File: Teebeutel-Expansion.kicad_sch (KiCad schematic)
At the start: 63 parts, among them J1 Conn_01x10_Male, J2 Conn_01x10_Female, J3 Conn_01x10_Male, J4 Conn_01x10_Female, J5 Conn_02x03_Counter_Clockwise, J6 Conn_02x03_Counter_Clockwise, J7 Conn_01x03, J8 Conn_01x03, J9 Conn_02x08_Counter_Clockwise

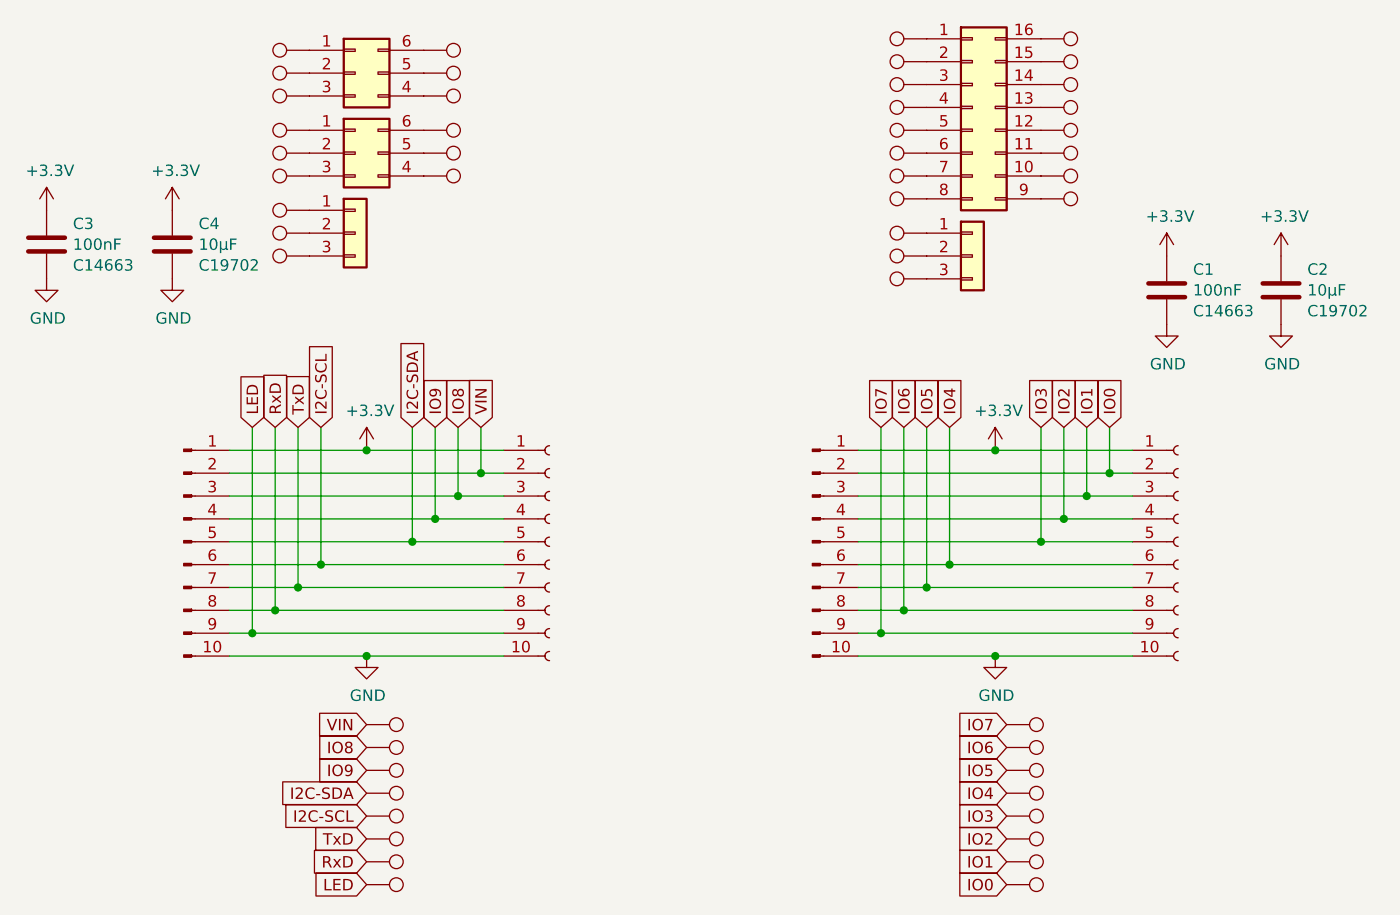
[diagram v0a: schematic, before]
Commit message: chore: Update labels
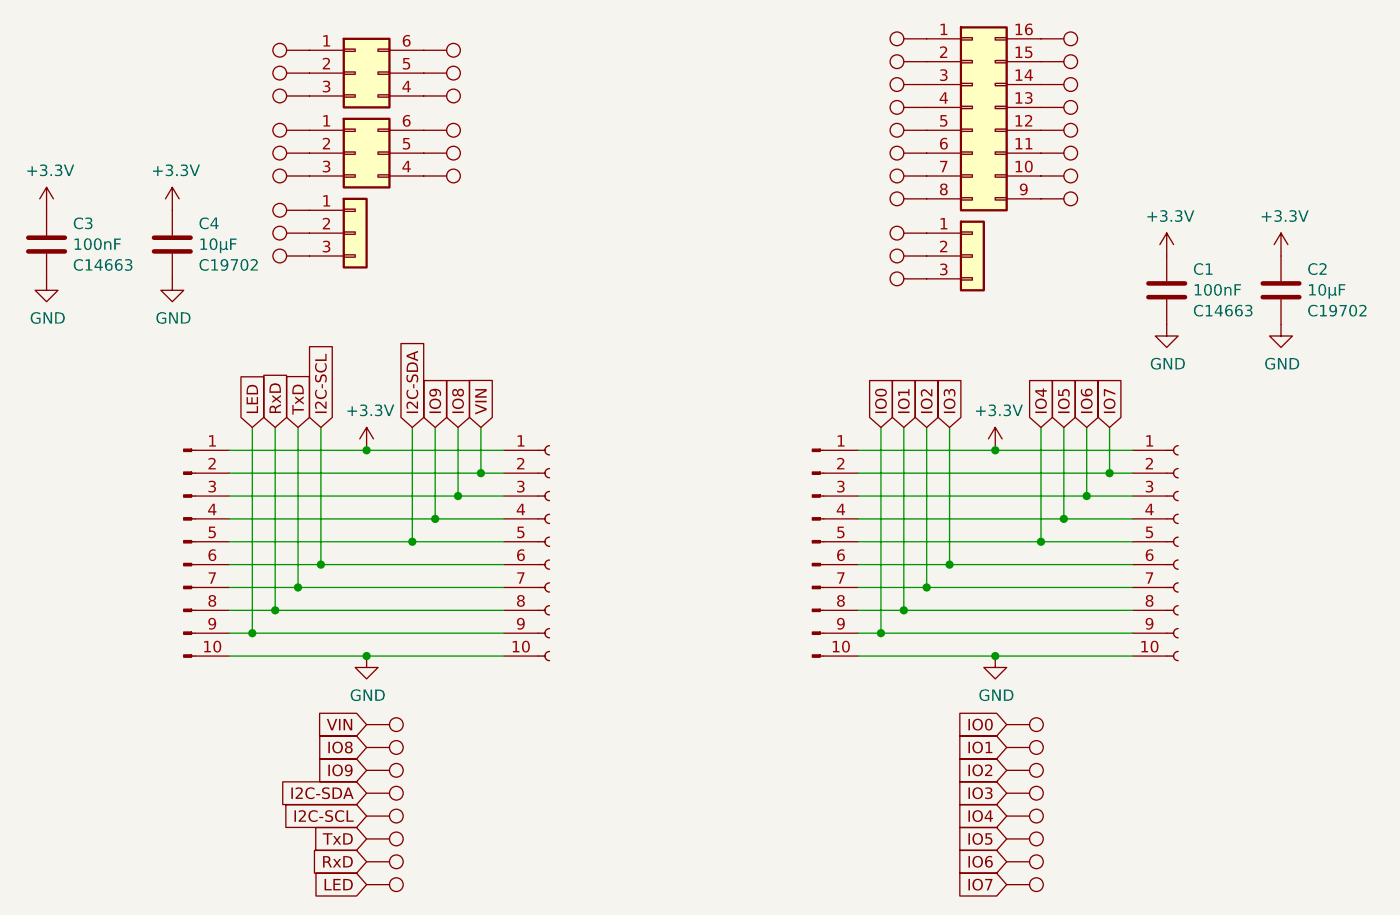
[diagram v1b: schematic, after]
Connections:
- net IO0: now also J3.9 (Pin_9), J4.9 (Pin_9), TP16.1; no longer J3.2 (Pin_2), J4.2 (Pin_2), TP9.1
- net IO1: now also J3.8 (Pin_8), J4.8 (Pin_8), TP15.1; no longer J3.3 (Pin_3), J4.3 (Pin_3), TP10.1
- net IO2: now also J3.7 (Pin_7), J4.7 (Pin_7), TP14.1; no longer J3.4 (Pin_4), J4.4 (Pin_4), TP11.1
- net IO3: now also J3.6 (Pin_6), J4.6 (Pin_6), TP13.1; no longer J3.5 (Pin_5), J4.5 (Pin_5), TP12.1
- net IO4: now also J3.5 (Pin_5), J4.5 (Pin_5), TP12.1; no longer J3.6 (Pin_6), J4.6 (Pin_6), TP13.1
- net IO5: now also J3.4 (Pin_4), J4.4 (Pin_4), TP11.1; no longer J3.7 (Pin_7), J4.7 (Pin_7), TP14.1
- net IO6: now also J3.3 (Pin_3), J4.3 (Pin_3), TP10.1; no longer J3.8 (Pin_8), J4.8 (Pin_8), TP15.1
- net IO7: now also J3.2 (Pin_2), J4.2 (Pin_2), TP9.1; no longer J3.9 (Pin_9), J4.9 (Pin_9), TP16.1
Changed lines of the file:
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@@
     )
   )
-  (global_label "IO7" (shape input) (at 182.88 123.19 180) (fields_autoplaced)
+  (global_label "IO7" (shape input) (at 182.88 140.97 180) (fields_autoplaced)
     (effects (font (size 1.27 1.27)) (justify right))
-    (property "Intersheet References" "${INTERSHEET_REFS}" (id 0) (at 0 0 0)
+    (property "Intersheet References" "${INTERSHEET_REFS}" (id 0) (at 0 264.16 0)
       (effects (font (size 1.27 1.27)) hide)
     )
   )
-  (global_label "IO6" (shape input) (at 171.45 90.17 90) (fields_autoplaced)
+  (global_label "IO6" (shape input) (at 191.77 90.17 90) (fields_autoplaced)
     (effects (font (size 1.27 1.27)) (justify left))
-    (property "Intersheet References" "${INTERSHEET_REFS}" (id 0) (at 0 0 0)
+    (property "Intersheet References" "${INTERSHEET_REFS}" (id 0) (at 363.22 0 0)
       (effects (font (size 1.27 1.27)) hide)
     )
@@
     )
   )
-  (global_label "IO7" (shape input) (at 168.91 90.17 90) (fields_autoplaced)
+  (global_label "IO7" (shape input) (at 194.31 90.17 90) (fields_autoplaced)
     (effects (font (size 1.27 1.27)) (justify left))
-    (property "Intersheet References" "${INTERSHEET_REFS}" (id 0) (at 0 0 0)
+    (property "Intersheet References" "${INTERSHEET_REFS}" (id 0) (at 363.22 0 0)
       (effects (font (size 1.27 1.27)) hide)
     )
@@
     )
   )
-  (global_label "IO5" (shape input) (at 182.88 128.27 180) (fields_autoplaced)
+  (global_label "IO5" (shape input) (at 182.88 135.89 180) (fields_autoplaced)
     (effects (font (size 1.27 1.27)) (justify right))
-    (property "Intersheet References" "${INTERSHEET_REFS}" (id 0) (at 0 0 0)
+    (property "Intersheet References" "${INTERSHEET_REFS}" (id 0) (at 0 264.16 0)
       (effects (font (size 1.27 1.27)) hide)
     )
@@
     )
   )
-  (global_label "IO4" (shape input) (at 182.88 130.81 180) (fields_autoplaced)
+  (global_label "IO4" (shape input) (at 182.88 133.35 180) (fields_autoplaced)
     (effects (font (size 1.27 1.27)) (justify right))
-    (property "Intersheet References" "${INTERSHEET_REFS}" (id 0) (at 0 0 0)
+    (property "Intersheet References" "${INTERSHEET_REFS}" (id 0) (at 0 264.16 0)
       (effects (font (size 1.27 1.27)) hide)
     )
   )
-  (global_label "IO2" (shape input) (at 182.88 135.89 180) (fields_autoplaced)
+  (global_label "IO2" (shape input) (at 182.88 128.27 180) (fields_autoplaced)
     (effects (font (size 1.27 1.27)) (justify right))
-    (property "Intersheet References" "${INTERSHEET_REFS}" (id 0) (at 0 0 0)
+    (property "Intersheet References" "${INTERSHEET_REFS}" (id 0) (at 0 264.16 0)
       (effects (font (size 1.27 1.27)) hide)
     )
@@
     )
   )
-  (global_label "IO5" (shape input) (at 173.99 90.17 90) (fields_autoplaced)
+  (global_label "IO5" (shape input) (at 189.23 90.17 90) (fields_autoplaced)
     (effects (font (size 1.27 1.27)) (justify left))
-    (property "Intersheet References" "${INTERSHEET_REFS}" (id 0) (at 0 0 0)
+    (property "Intersheet References" "${INTERSHEET_REFS}" (id 0) (at 363.22 0 0)
       (effects (font (size 1.27 1.27)) hide)
     )
@@
     )
   )
-  (global_label "IO2" (shape input) (at 189.23 90.17 90) (fields_autoplaced)
+  (global_label "IO2" (shape input) (at 173.99 90.17 90) (fields_autoplaced)
     (effects (font (size 1.27 1.27)) (justify left))
-    (property "Intersheet References" "${INTERSHEET_REFS}" (id 0) (at 0 0 0)
+    (property "Intersheet References" "${INTERSHEET_REFS}" (id 0) (at 363.22 0 0)
       (effects (font (size 1.27 1.27)) hide)
     )
@@
     )
   )
-  (global_label "IO6" (shape input) (at 182.88 125.73 180) (fields_autoplaced)
+  (global_label "IO6" (shape input) (at 182.88 138.43 180) (fields_autoplaced)
     (effects (font (size 1.27 1.27)) (justify right))
-    (property "Intersheet References" "${INTERSHEET_REFS}" (id 0) (at 0 0 0)
+    (property "Intersheet References" "${INTERSHEET_REFS}" (id 0) (at 0 264.16 0)
       (effects (font (size 1.27 1.27)) hide)
     )
   )
-  (global_label "IO3" (shape input) (at 186.69 90.17 90) (fields_autoplaced)
+  (global_label "IO3" (shape input) (at 176.53 90.17 90) (fields_autoplaced)
     (effects (font (size 1.27 1.27)) (justify left))
-    (property "Intersheet References" "${INTERSHEET_REFS}" (id 0) (at 0 0 0)
+    (property "Intersheet References" "${INTERSHEET_REFS}" (id 0) (at 363.22 0 0)
       (effects (font (size 1.27 1.27)) hide)
     )
   )
-  (global_label "IO4" (shape input) (at 176.53 90.17 90) (fields_autoplaced)
+  (global_label "IO4" (shape input) (at 186.69 90.17 90) (fields_autoplaced)
     (effects (font (size 1.27 1.27)) (justify left))
-    (property "Intersheet References" "${INTERSHEET_REFS}" (id 0) (at 0 0 0)
+    (property "Intersheet References" "${INTERSHEET_REFS}" (id 0) (at 363.22 0 0)
       (effects (font (size 1.27 1.27)) hide)
     )
@@
     )
   )
-  (global_label "IO1" (shape input) (at 182.88 138.43 180) (fields_autoplaced)
+  (global_label "IO1" (shape input) (at 182.88 125.73 180) (fields_autoplaced)
     (effects (font (size 1.27 1.27)) (justify right))
-    (property "Intersheet References" "${INTERSHEET_REFS}" (id 0) (at 0 0 0)
+    (property "Intersheet References" "${INTERSHEET_REFS}" (id 0) (at 0 264.16 0)
       (effects (font (size 1.27 1.27)) hide)
     )
   )
-  (global_label "IO1" (shape input) (at 191.77 90.17 90) (fields_autoplaced)
+  (global_label "IO1" (shape input) (at 171.45 90.17 90) (fields_autoplaced)
     (effects (font (size 1.27 1.27)) (justify left))
-    (property "Intersheet References" "${INTERSHEET_REFS}" (id 0) (at 0 0 0)
+    (property "Intersheet References" "${INTERSHEET_REFS}" (id 0) (at 363.22 0 0)
       (effects (font (size 1.27 1.27)) hide)
     )
   )
-  (global_label "IO3" (shape input) (at 182.88 133.35 180) (fields_autoplaced)
+  (global_label "IO3" (shape input) (at 182.88 130.81 180) (fields_autoplaced)
     (effects (font (size 1.27 1.27)) (justify right))
-    (property "Intersheet References" "${INTERSHEET_REFS}" (id 0) (at 0 0 0)
+    (property "Intersheet References" "${INTERSHEET_REFS}" (id 0) (at 0 264.16 0)
       (effects (font (size 1.27 1.27)) hide)
     )
   )
-  (global_label "IO0" (shape input) (at 194.31 90.17 90) (fields_autoplaced)
+  (global_label "IO0" (shape input) (at 168.91 90.17 90) (fields_autoplaced)
     (effects (font (size 1.27 1.27)) (justify left))
-    (property "Intersheet References" "${INTERSHEET_REFS}" (id 0) (at 0 0 0)
+    (property "Intersheet References" "${INTERSHEET_REFS}" (id 0) (at 363.22 0 0)
       (effects (font (size 1.27 1.27)) hide)
     )
   )
-  (global_label "IO0" (shape input) (at 182.88 140.97 180) (fields_autoplaced)
+  (global_label "IO0" (shape input) (at 182.88 123.19 180) (fields_autoplaced)
     (effects (font (size 1.27 1.27)) (justify right))
-    (property "Intersheet References" "${INTERSHEET_REFS}" (id 0) (at 0 0 0)
+    (property "Intersheet References" "${INTERSHEET_REFS}" (id 0) (at 0 264.16 0)
       (effects (font (size 1.27 1.27)) hide)
     )
